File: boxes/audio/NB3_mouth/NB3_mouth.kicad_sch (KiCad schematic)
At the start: 4 parts, among them IC1 MAX98357AETE+T, J1 Conn_02x03_Odd_Even, J2 Conn_02x03_Odd_Even, J3 JST-PH2

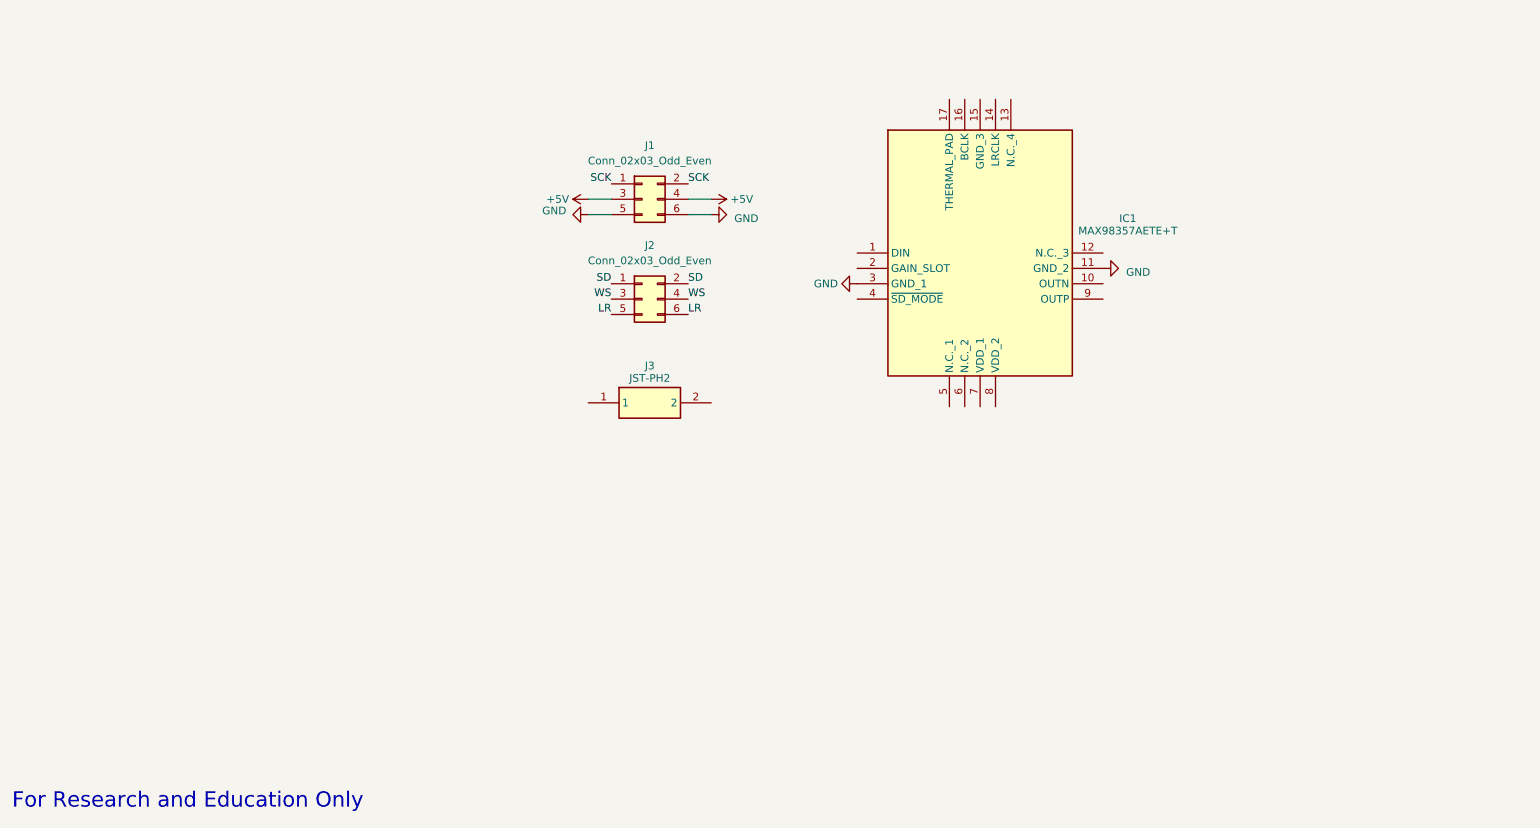
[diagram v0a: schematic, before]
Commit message: Upload NB3_ear "fab" v2
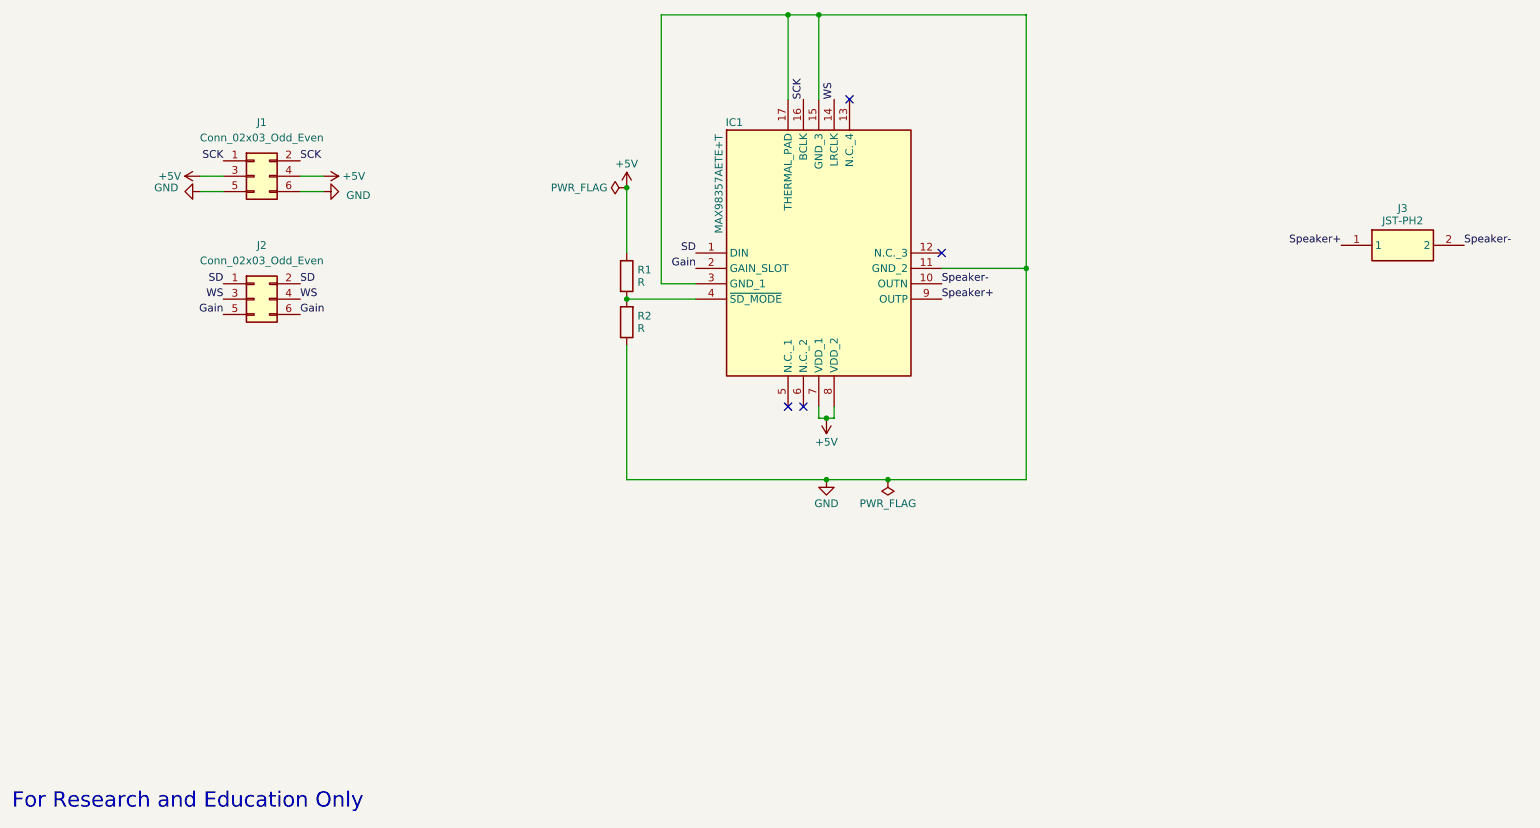
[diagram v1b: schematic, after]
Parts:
- added R1, R2: R, Resistor_SMD:R_0402_1005Metric, symbol Device:R
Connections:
- net LR is gone; now on net Gain: J2.5 (Pin_5), J2.6 (Pin_6)
- net +5V: now also IC1.7 (VDD_1), IC1.8 (VDD_2), R1.1
- net GND: now also IC1.15 (GND_3), IC1.17 (THERMAL_PAD), R2.1
- net SCK: now also IC1.16 (BCLK)
- net SD: now also IC1.1 (DIN)
- net WS: now also IC1.14 (LRCLK)
- net Speaker-: now reaches IC1.10 (OUTN)
- net Speaker-: now also J3.2
- net Gain: now reaches IC1.2 (GAIN_SLOT)
- net at IC1.4 (~{SD_MODE}): now also R1.2, R2.2
- net Speaker+: now reaches IC1.9 (OUTP)
- net Speaker+: now also J3.1
- no-connect marks 0 -> 4
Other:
- moved on the sheet: IC1, J1, J2, J3
